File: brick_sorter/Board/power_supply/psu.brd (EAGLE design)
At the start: 51.5 x 60.4 mm, 14 parts, among them IC1 LM2574N-3.3, IC2-12V 786TV, IC2-6V 786TV

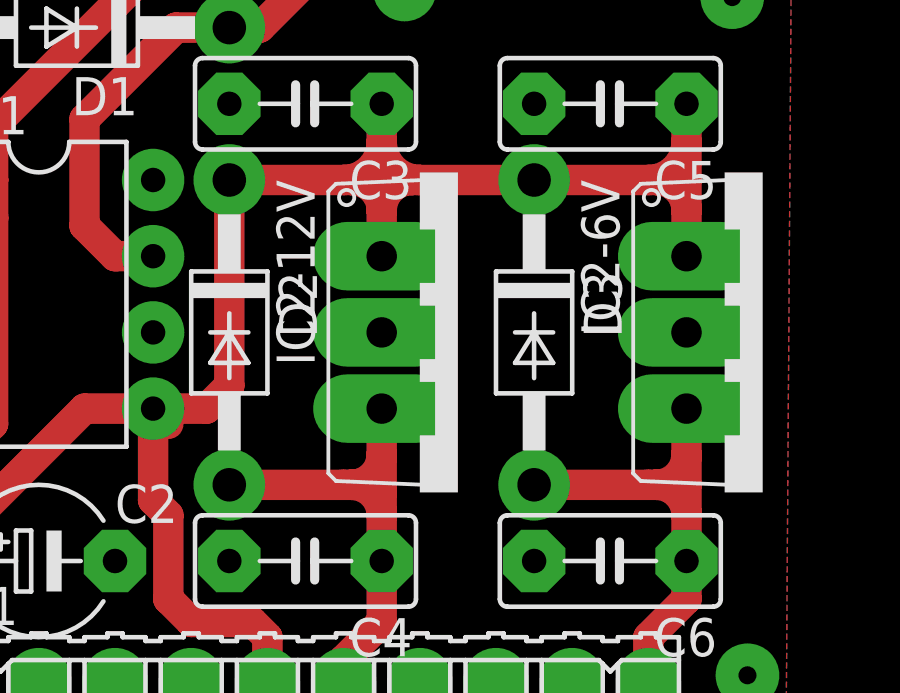
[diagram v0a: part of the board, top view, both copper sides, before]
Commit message: Updates to report
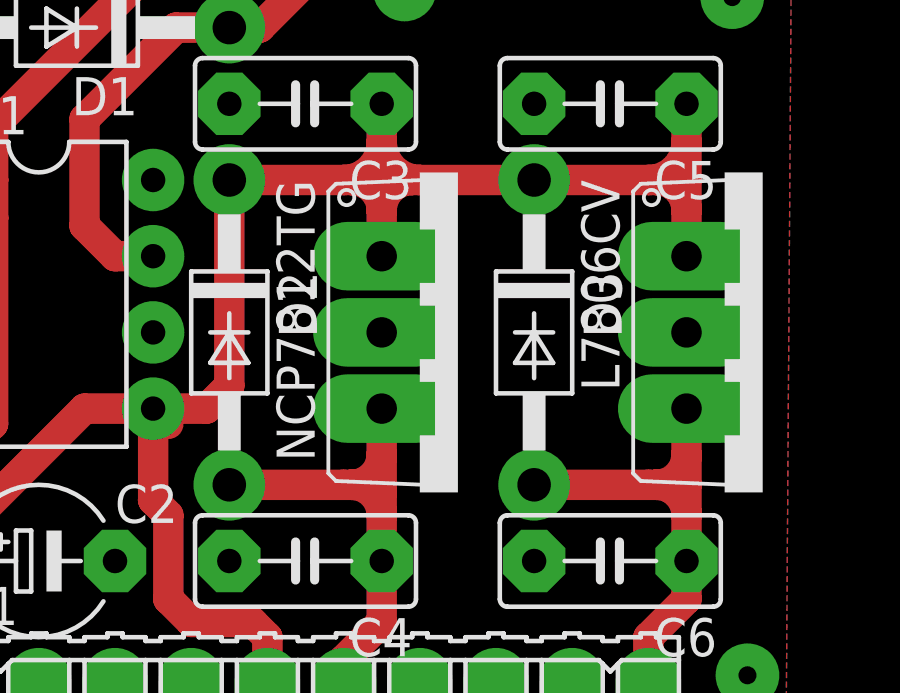
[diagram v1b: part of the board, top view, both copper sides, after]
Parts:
- C1: value (none) -> 330uF
- C2: value (none) -> 22uF
- C3, C4, C5, C6: value (none) -> 330nF
- D1: value BYV10 -> 1N5817
- L1: value (none) -> 330uH
- renumbered IC2-12V to NCP7812TG, IC2-6V to L7806CV
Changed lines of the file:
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@@
 </autorouter>
 <elements>
-<element name="C1" library="rcl" package="E5-8,5" value="" x="22.86" y="43.688" rot="R180"/>
-<element name="C2" library="rcl" package="E5-5" value="" x="16.51" y="19.558"/>
-<element name="C3" library="rcl" package="C050-030X075" value="" x="25.4" y="34.798" rot="R180"/>
-<element name="C4" library="rcl" package="C050-030X075" value="" x="25.4" y="19.558" rot="R180"/>
-<element name="C5" library="rcl" package="C050-030X075" value="" x="35.56" y="34.798" rot="R180"/>
-<element name="C6" library="rcl" package="C050-030X075" value="" x="35.56" y="19.558" rot="R180"/>
-<element name="D1" library="diode" package="DO41-10" value="BYV10" x="17.78" y="37.338" rot="R180"/>
+<element name="C1" library="rcl" package="E5-8,5" value="330uF" x="22.86" y="43.688" rot="R180"/>
+<element name="C2" library="rcl" package="E5-5" value="22uF" x="16.51" y="19.558"/>
+<element name="C3" library="rcl" package="C050-030X075" value="330nF" x="25.4" y="34.798" rot="R180"/>
+<element name="C4" library="rcl" package="C050-030X075" value="330nF" x="25.4" y="19.558" rot="R180"/>
+<element name="C5" library="rcl" package="C050-030X075" value="330nF" x="35.56" y="34.798" rot="R180"/>
+<element name="C6" library="rcl" package="C050-030X075" value="330nF" x="35.56" y="19.558" rot="R180"/>
+<element name="D1" library="diode" package="DO41-10" value="1N5817" x="17.78" y="37.338" rot="R180"/>
 <element name="D2" library="diode" package="DO41-10" value="1N4004" x="22.86" y="27.178" rot="R270"/>
 <element name="D3" library="diode" package="DO41-10" value="1N4004" x="33.02" y="27.178" rot="R270"/>
 <element name="IC1" library="linear" package="DIL08" value="LM2574N-3.3" x="16.51" y="28.448" rot="R270"/>
-<element name="IC2-12V" library="linear" package="TO220V" value="786TV" x="30.48" y="27.178" rot="R270"/>
-<element name="IC2-6V" library="linear" package="TO220V" value="786TV" x="40.64" y="27.178" rot="R270"/>
+<element name="NCP7812TG" library="linear" package="TO220V" value="786TV" x="30.48" y="27.178" rot="R270"/>
+<element name="L7806CV" library="linear" package="TO220V" value="786TV" x="40.64" y="27.178" rot="R270"/>
 <element name="SL1" library="con-amp-quick" package="10P" value="" x="25.4" y="14.478">
 <attribute name="MF" value="" x="25.4" y="14.478" size="1.778" layer="27" display="off"/>
@@
 <attribute name="MPN" value="" x="25.4" y="14.478" size="1.778" layer="27" display="off"/>
 </element>
-<element name="L1" library="inductor-neosid" package="BS11" value="" x="74.168" y="41.656">
+<element name="L1" library="inductor-neosid" package="BS11" value="330uH" x="74.168" y="41.656">
 <attribute name="MPN" value="" x="74.168" y="41.656" size="1.778" layer="27" display="off"/>
 <attribute name="MF" value="" x="74.168" y="41.656" size="1.778" layer="27" display="off"/>
@@
 <contactref element="C2" pad="+"/>
 <contactref element="IC1" pad="5"/>
-<contactref element="IC2-12V" pad="1"/>
+<contactref element="NCP7812TG" pad="1"/>
 <contactref element="C3" pad="1"/>
 <contactref element="D2" pad="C"/>
-<contactref element="IC2-6V" pad="1"/>
+<contactref element="L7806CV" pad="1"/>
 <contactref element="C5" pad="1"/>
 <contactref element="D3" pad="C"/>
@@
 <contactref element="C1" pad="-"/>
 <contactref element="D1" pad="A"/>
-<contactref element="IC2-12V" pad="2"/>
+<contactref element="NCP7812TG" pad="2"/>
 <contactref element="C3" pad="2"/>
 <contactref element="C4" pad="2"/>
-<contactref element="IC2-6V" pad="2"/>
+<contactref element="L7806CV" pad="2"/>
 <contactref element="C5" pad="2"/>
 <contactref element="C6" pad="2"/>
@@
 </signal>
 <signal name="6V">
-<contactref element="IC2-6V" pad="3"/>
+<contactref element="L7806CV" pad="3"/>
 <contactref element="C6" pad="1"/>
 <contactref element="D3" pad="A"/>
@@
 </signal>
 <signal name="12V">
-<contactref element="IC2-12V" pad="3"/>
+<contactref element="NCP7812TG" pad="3"/>
 <contactref element="C4" pad="1"/>
 <contactref element="D2" pad="A"/>
